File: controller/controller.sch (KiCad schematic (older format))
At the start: 65 parts, among them J1 Conn_01x25_Membrane, J2 Conn_01x04, J3 Conn_Solenoid_Driver, J4 Conn_01x01, J6 Conn_01x06, Q1 Q_PMOS_GSD AO3401A, Q2 Q_NMOS_GSD 2N7002, Q3 Q_NMOS_GSD 2N7002, SW1 SW_Push, U1 AMS1117-3.3, U2 STM32F446RETx, U3 TPS2553DBVR, U4 USBLC6-2SC6, U5 24LC64, Y1 16MHz

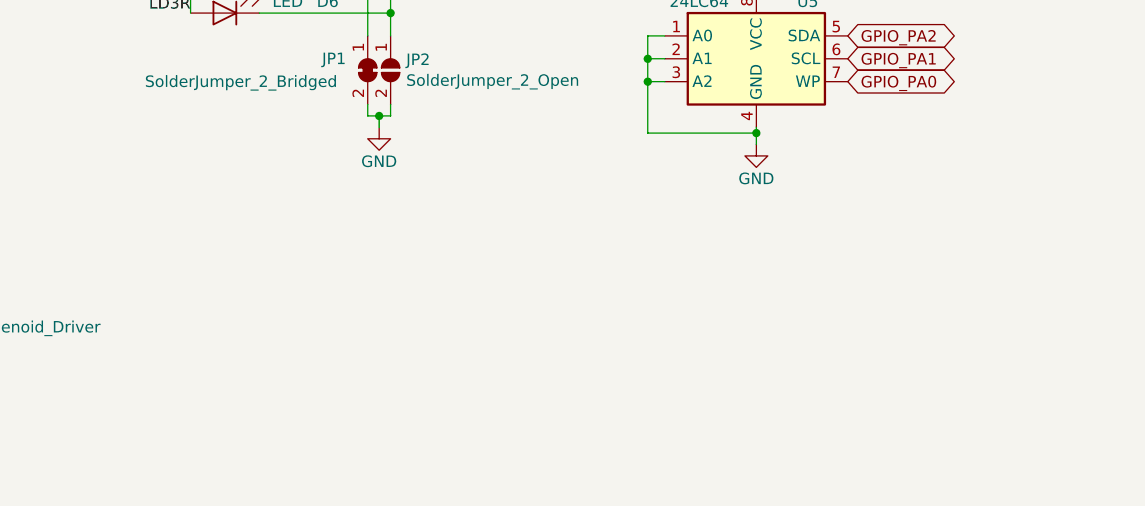
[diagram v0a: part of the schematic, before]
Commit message: Prepare the design for release
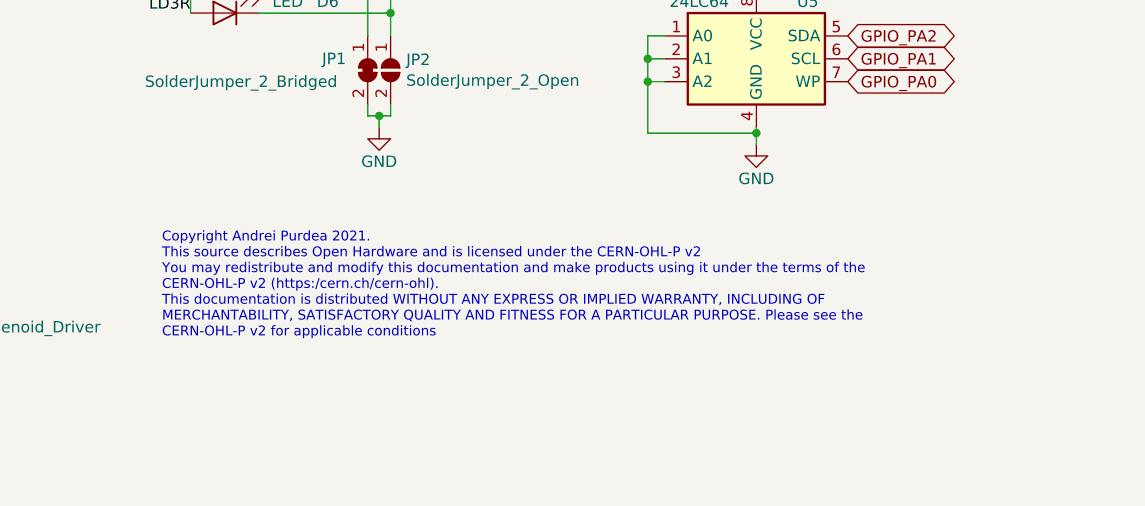
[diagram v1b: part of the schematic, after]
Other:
- note added: "Copyright Andrei Purdea 2021.\nThis source describes Open Hardware and is licensed under the CERN-OHL-P v2\nYou may redistribute and modify this documentation and make products using it under the terms of the\nCERN-OHL-P v2 (https:/cern.ch/cern-ohl).\nThis documentation is distributed WITHOUT ANY EXPRESS OR IMPLIED WARRANTY, INCLUDING OF\nMERCHANTABILITY, SATISFACTORY QUALITY AND FITNESS FOR A PA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"
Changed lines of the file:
@@
 encoding utf-8
 Sheet 1 1
-Title ""
+Title "OverNumpad Controller"
 Date ""
 Rev ""
@@
 NoConn ~ 1450 3725
 NoConn ~ 1650 4225
+Text Notes 7025 7075 0    43   ~ 0
+Copyright Andrei Purdea 2021.\nThis source describes Open Hardware and is licensed under the CERN-OHL-P v2\nYou may redistribute and modify this documentation and make products using it under the terms of the\nCERN-OHL-P v2 (https:/cern.ch/cern-ohl).\nThis documentation is distributed WITHOUT ANY EXPRESS OR IMPLIED WARRANTY, INCLUDING OF\nMERCHANTABILITY, SATISFACTORY QUALITY AND FITNESS FOR A PARTICULAR PURPOSE. Please see the\nCERN-OHL-P v2 for applicable conditions
 $EndSCHEMATC
